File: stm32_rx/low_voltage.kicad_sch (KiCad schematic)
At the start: 0 parts

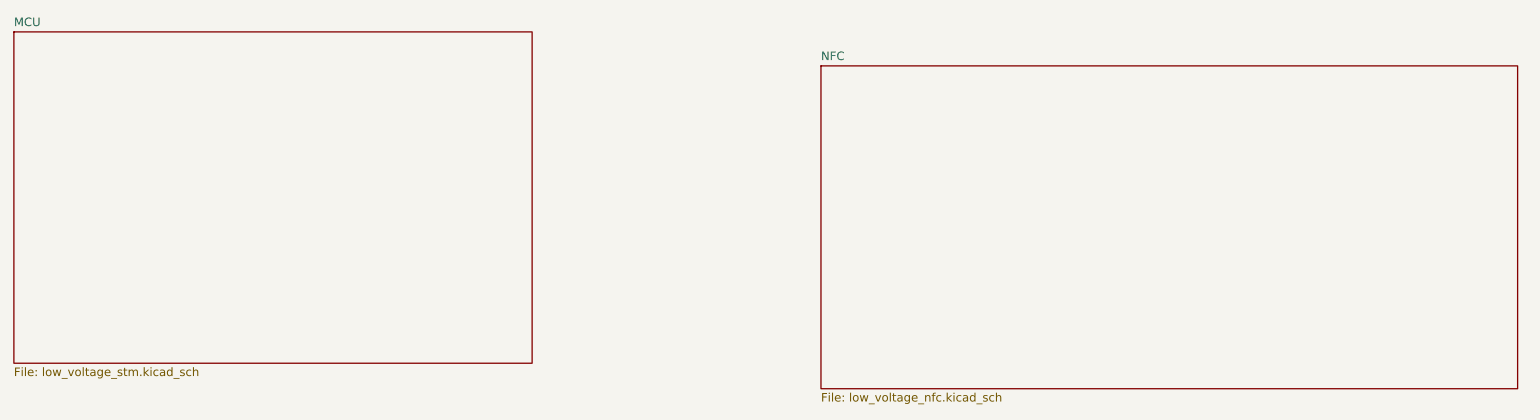
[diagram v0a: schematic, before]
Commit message: I can't find the right module
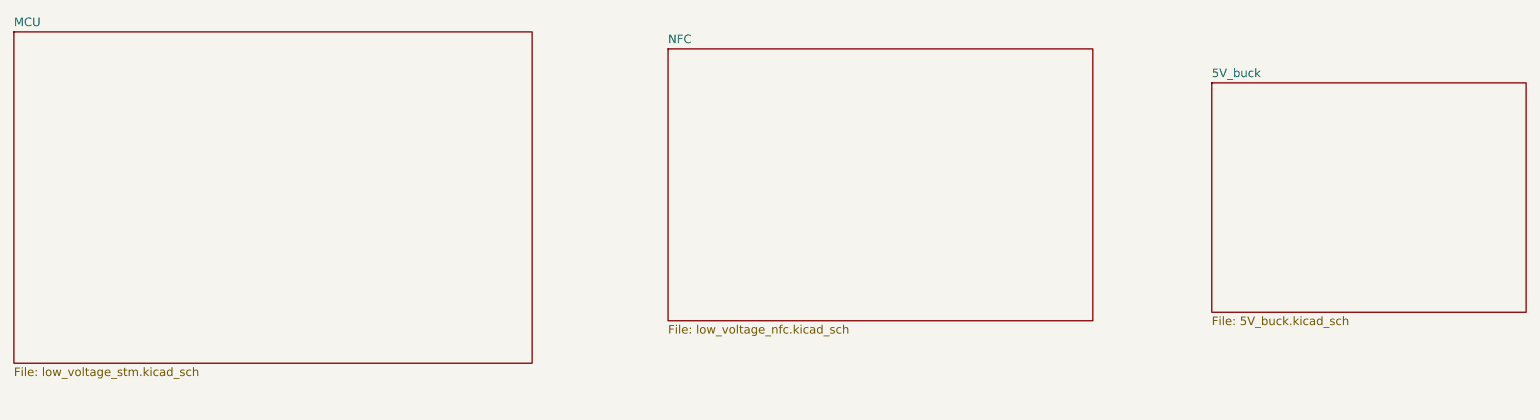
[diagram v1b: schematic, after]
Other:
- added sheet 5V_buck (5V_buck.kicad_sch)
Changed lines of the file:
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@@
 	(paper "A4")
+	(sheet
+		(at 215.9 85.09)
+		(size 46.99 34.29)
+		(exclude_from_sim no)
+		(in_bom yes)
+		(on_board yes)
+		(dnp no)
+		(fields_autoplaced yes)
+		(stroke
+			(width 0.1524)
+			(type solid)
+		)
+		(fill
+			(color 0 0 0 0.0000)
+		)
+		(property "Sheetname" "5V_buck"
+			(at 215.9 84.3784 0)
+			(effects
+				(font
+					(size 1.27 1.27)
+				)
+				(justify left bottom)
+			)
+		)
+		(property "Sheetfile" "5V_buck.kicad_sch"
+			(at 215.9 119.9646 0)
+			(effects
+				(font
+					(size 1.27 1.27)
+				)
+				(justify left top)
+			)
+		)
+		(property "Field2" ""
+			(at 215.9 85.09 0)
+			(effects
+				(font
+					(size 1.27 1.27)
+				)
+			)
+		)
+		(instances
+			(project "stm32_rx"
+				(path "/df2eee68-9211-4709-aa52-0070953818c3/0796e7dd-f836-4c1c-8676-47f22f9cd6a5"
+					(page "8")
+				)
+			)
+		)
+	)
 	(sheet
 		(at 36.83 77.47)
@@
 	)
 	(sheet
-		(at 157.48 82.55)
-		(size 104.14 48.26)
+		(at 134.62 80.01)
+		(size 63.5 40.64)
 		(exclude_from_sim no)
 		(in_bom yes)
@@
 		)
 		(property "Sheetname" "NFC"
-			(at 157.48 81.8384 0)
+			(at 134.62 79.2984 0)
 			(effects
 				(font
@@
 		)
 		(property "Sheetfile" "low_voltage_nfc.kicad_sch"
-			(at 157.48 131.3946 0)
+			(at 134.62 121.2346 0)
 			(effects
 				(font
